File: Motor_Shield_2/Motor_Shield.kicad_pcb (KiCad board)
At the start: 2 copper layers, 59.1 x 64.8 mm, 49 parts, among them J1 Conn_01x08_Female, J10 Conn_01x02_Male, J11 Conn_01x02_Male, J12 Conn_01x02_Male, J13 Conn_01x02_Male, J14 Conn_01x02_Male, J15 Conn_01x02_Male, J16 Conn_01x02_Male, J17 Conn_01x02_Male, J18 Conn_01x02_Male, J19 Conn_01x02_Male, J2 Conn_01x06_Female, J20 Conn_01x02_Male, J21 Conn_01x02_Male, J22 Conn_01x02_Male, J3 Conn_01x08_Female, J4 Conn_01x10_Female, J5 Conn_01x02_Female, J6 Screw_Terminal_01x06, J7 Conn_01x02_Male, J8 Conn_01x02_Male, J9 Conn_01x02_Male, U1 L6474PD

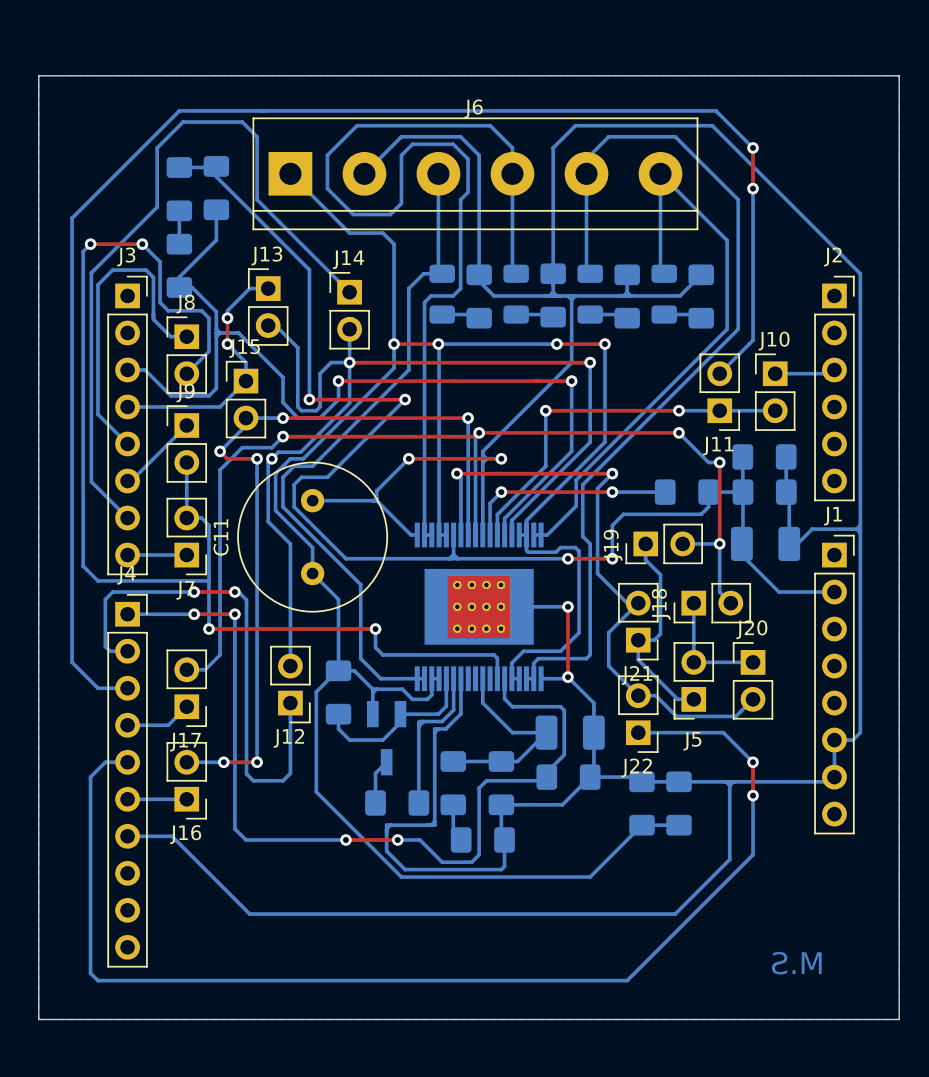
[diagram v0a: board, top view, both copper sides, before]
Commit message: Überarbeiten das Pin Header schlecht plaziert waren
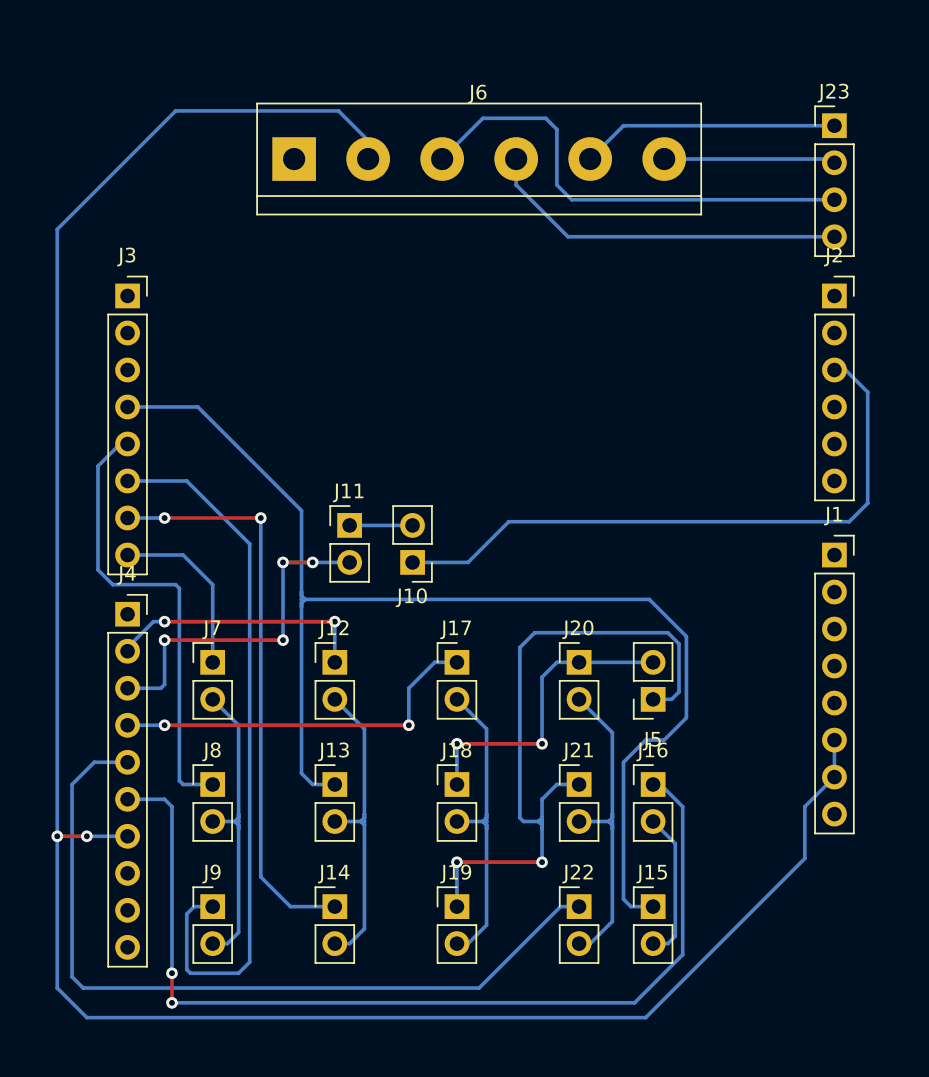
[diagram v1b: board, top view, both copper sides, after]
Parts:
- removed C1: 3.3nF, Capacitor_SMD:C_1206_3216Metric_Pad1.42x1.75mm_HandSolder
- removed C10, C2, C4, C5, C9: 100nF, Capacitor_SMD:C_1206_3216Metric_Pad1.42x1.75mm_HandSolder
- removed C11: 100uF 63V, Capacitor_THT:C_Radial_D10.0mm_H20.0mm_P5.00mm
- removed C3: 47uF, Capacitor_Tantalum_SMD:CP_EIA-3528-12_Kemet-T_Pad1.50x2.35mm_HandSolder
- removed C6: 10uF, Capacitor_Tantalum_SMD:CP_EIA-3528-12_Kemet-T_Pad1.50x2.35mm_HandSolder
- removed C7: 220nF, Capacitor_SMD:C_1206_3216Metric_Pad1.42x1.75mm_HandSolder
- removed C8: 10nF, Capacitor_SMD:C_1206_3216Metric_Pad1.42x1.75mm_HandSolder
- removed D1, D2: LED, Diode_SMD:D_1206_3216Metric_Pad1.42x1.75mm_HandSolder
- removed D3: D_Schottky_x2_Serial_AKC, Package_TO_SOT_SMD:SC-59_Handsoldering
- removed D4, D5, D6, D7: LED, Diode_SMD:D_1206_3216Metric
- removed R1, R18: 330, Resistor_SMD:R_1206_3216Metric_Pad1.42x1.75mm_HandSolder
- removed R14, R2: 10k, Resistor_SMD:R_1206_3216Metric_Pad1.42x1.75mm_HandSolder
- removed R22, R23, R24, R25: 2.2k, Resistor_SMD:R_1206_3216Metric_Pad1.42x1.75mm_HandSolder
- removed U1: L6474PD, Package_SO:ST_PowerSSO-36_SlugDown_ThermalVias
- added J23: Conn_01x04_Female, Connector_PinHeader_2.54mm:PinHeader_1x04_P2.54mm_Vertical, F.Cu at (175.3, 62.5)
- moved J15 45.6 mm to (162.8, 116.1)
- moved J14 42.2 mm to (141.0, 116.1)
- moved J13 34.3 mm to (141.0, 107.7)
- moved J9 33.1 mm to (132.6, 116.1)
- moved J16 32.0 mm to (162.8, 107.7), turned to 0 degrees
- moved J8 30.8 mm to (132.6, 107.7)
- moved J10 28.1 mm to (146.3, 92.5), turned to 180 degrees
- moved J19 28.1 mm to (149.4, 116.1), turned to 0 degrees
- moved J11 26.6 mm to (142.0, 89.9), turned to 0 degrees
- moved J18 20.5 mm to (149.4, 107.7), turned to 0 degrees
- moved J17 18.8 mm to (149.4, 99.3), turned to 0 degrees
- moved J22 12.6 mm to (157.7, 116.1), turned to 0 degrees
- moved J20 11.9 mm to (157.7, 99.3)
- moved J21 10.7 mm to (157.7, 107.7), turned to 0 degrees
- moved J7 7.58 mm to (132.6, 99.3), turned to 0 degrees
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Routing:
- net VS: track 154.4 -> 0.00 mm, vias 4 -> 0
- net GND: track 291.2 -> 149.4 mm, vias 4 -> 2
- net VDD: track 91.8 -> 0.00 mm, vias 4 -> 0
- net Net-(J11-Pad2): track 102.6 -> 23.7 mm, vias 2 -> 4
- net Net-(J13-Pad1): track 17.6 -> 87.0 mm, vias 2 -> 0
- net Net-(D1-Pad1): track 65.0 -> 0.00 mm, vias 2 -> 0
- net Net-(J16-Pad1): track 3.56 -> 66.0 mm, vias 0 -> 2
- net Net-(J7-Pad2): track 83.1 -> 21.8 mm, vias 4 -> 0
- net Net-(C2-Pad1): track 60.4 -> 0.00 mm, vias 4 -> 0
- net Net-(J17-Pad2): track 71.5 -> 22.2 mm, vias 5 -> 0
- net Net-(J12-Pad2): track 70.6 -> 22.0 mm, vias 3 -> 0
- net Net-(J23-Pad1): track 62.4 -> 17.7 mm
- net Net-(J15-Pad2): track 54.7 -> 10.2 mm, vias 6 -> 0
- net Net-(J3-Pad6): track 5.64 -> 49.4 mm
- net Net-(J23-Pad4): track 68.4 -> 25.1 mm
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- removed copper zone on B.Cu, net GND
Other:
- board outline removed
- board text removed: "M.S"

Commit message: PCB fertig
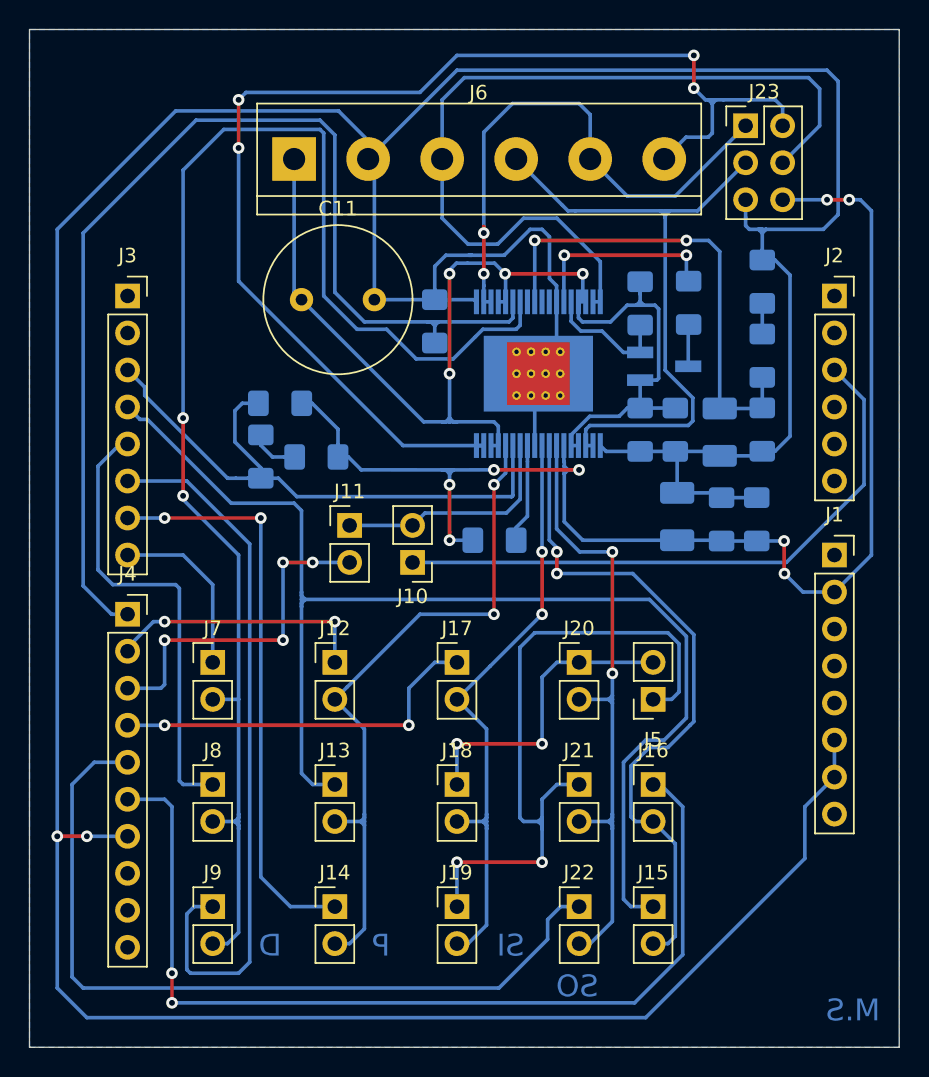
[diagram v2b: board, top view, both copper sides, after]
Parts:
- added C1: 3.3nF, Capacitor_SMD:C_1206_3216Metric_Pad1.42x1.75mm_HandSolder, B.Cu at (169.9, 89.5)
- added C10: 100nF, Capacitor_SMD:C_1206_3216Metric_Pad1.42x1.75mm_HandSolder, B.Cu at (161.9, 83.3)
- added C11: 100uF 63V, Capacitor_THT:C_Radial_D10.0mm_H20.0mm_P5.00mm, F.Cu at (138.7, 74.4)
- added C2: 100nF, Capacitor_SMD:C_1206_3216Metric_Pad1.42x1.75mm_HandSolder, B.Cu at (147.8, 75.9)
- added C3: 47uF, Capacitor_Tantalum_SMD:CP_EIA-3528-12_Kemet-T_Pad1.50x2.35mm_HandSolder, B.Cu at (167.4, 83.5)
- added C4: 100nF, Capacitor_SMD:C_1206_3216Metric_Pad1.42x1.75mm_HandSolder, B.Cu at (167.5, 89.5)
- added C5: 100nF, Capacitor_SMD:C_1206_3216Metric_Pad1.42x1.75mm_HandSolder, B.Cu at (170.3, 83.3)
- added C6: 10uF, Capacitor_Tantalum_SMD:CP_EIA-3528-12_Kemet-T_Pad1.50x2.35mm_HandSolder, B.Cu at (164.5, 89.3)
- added C7: 220nF, Capacitor_SMD:C_1206_3216Metric_Pad1.42x1.75mm_HandSolder, B.Cu at (161.9, 74.7)
- added C8: 10nF, Capacitor_SMD:C_1206_3216Metric_Pad1.42x1.75mm_HandSolder, B.Cu at (165.3, 74.6)
- added C9: 100nF, Capacitor_SMD:C_1206_3216Metric_Pad1.42x1.75mm_HandSolder, B.Cu at (164.3, 83.3)
- added D1: LED, Diode_SMD:D_1206_3216Metric_Pad1.42x1.75mm_HandSolder, B.Cu at (135.9, 85.2)
- added D2: LED, Diode_SMD:D_1206_3216Metric_Pad1.42x1.75mm_HandSolder, B.Cu at (170.3, 73.2)
- added D3: D_Schottky_x2_Serial_AKC, Package_TO_SOT_SMD:SC-59_Handsoldering, B.Cu at (163.6, 79.0)
- added R1: 330, Resistor_SMD:R_1206_3216Metric_Pad1.42x1.75mm_HandSolder, B.Cu at (139.7, 85.2)
- added R14: 10k, Resistor_SMD:R_1206_3216Metric_Pad1.42x1.75mm_HandSolder, B.Cu at (151.9, 90.9)
- added R18: 330, Resistor_SMD:R_1206_3216Metric_Pad1.42x1.75mm_HandSolder, B.Cu at (170.3, 78.3)
- added R2: 10k, Resistor_SMD:R_1206_3216Metric_Pad1.42x1.75mm_HandSolder, B.Cu at (137.2, 81.5)
- added U1: L6474PD, Package_SO:ST_PowerSSO-36_SlugDown_ThermalVias, B.Cu at (154.9, 79.5)
- J23: value Conn_01x04_Female -> Conn_02x03_Counter_Clockwise; footprint Connector_PinHeader_2.54mm:PinHeader_1x04_P2.54mm_Vertical -> Connector_PinHeader_2.54mm:PinHeader_2x03_P2.54mm_Vertical
- moved J23 6.10 mm to (169.2, 62.5)
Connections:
- J6 pad 3: Net-(J23-Pad3) -> Net-(J23-Pad4)
- J6 pad 4: Net-(J23-Pad4) -> Net-(J23-Pad3)
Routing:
- net GND: track 149.4 -> 285.5 mm
- net VDD: track 0.00 -> 91.9 mm, vias 0 -> 8
- net VS: track 0.00 -> 82.5 mm, vias 0 -> 4
- net Net-(J7-Pad2): track 21.8 -> 100.7 mm, vias 0 -> 2
- net Net-(C2-Pad1): track 0.00 -> 76.5 mm
- net Net-(J23-Pad2): track 11.8 -> 84.1 mm, vias 0 -> 4
- net Net-(D1-Pad1): track 0.00 -> 41.1 mm
- net Net-(J15-Pad2): track 10.2 -> 47.1 mm, vias 0 -> 2
- net Net-(C3-Pad1): track 0.00 -> 33.0 mm, vias 0 -> 2
- net Net-(J23-Pad4): track 25.1 -> 57.9 mm
- net Net-(J12-Pad2): track 22.0 -> 47.3 mm, vias 0 -> 2
- net Net-(J20-Pad2): track 22.6 -> 45.0 mm, vias 0 -> 2
- net Net-(J23-Pad1): track 17.7 -> 38.2 mm, vias 0 -> 2
- net Net-(J17-Pad2): track 22.2 -> 42.0 mm, vias 0 -> 2
- net Net-(C8-Pad2): track 0.00 -> 13.4 mm, vias 0 -> 2
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- added copper zone on B.Cu, net GND
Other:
- board outline added: 59.7 x 69.8 mm
- board text added: "D"
- board text added: "M.S"
- board text added: "P"
- board text added: "SI"
- board text added: "SO"
